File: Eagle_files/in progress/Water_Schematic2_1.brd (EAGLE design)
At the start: 26.4 x 45.5 mm, 10 parts

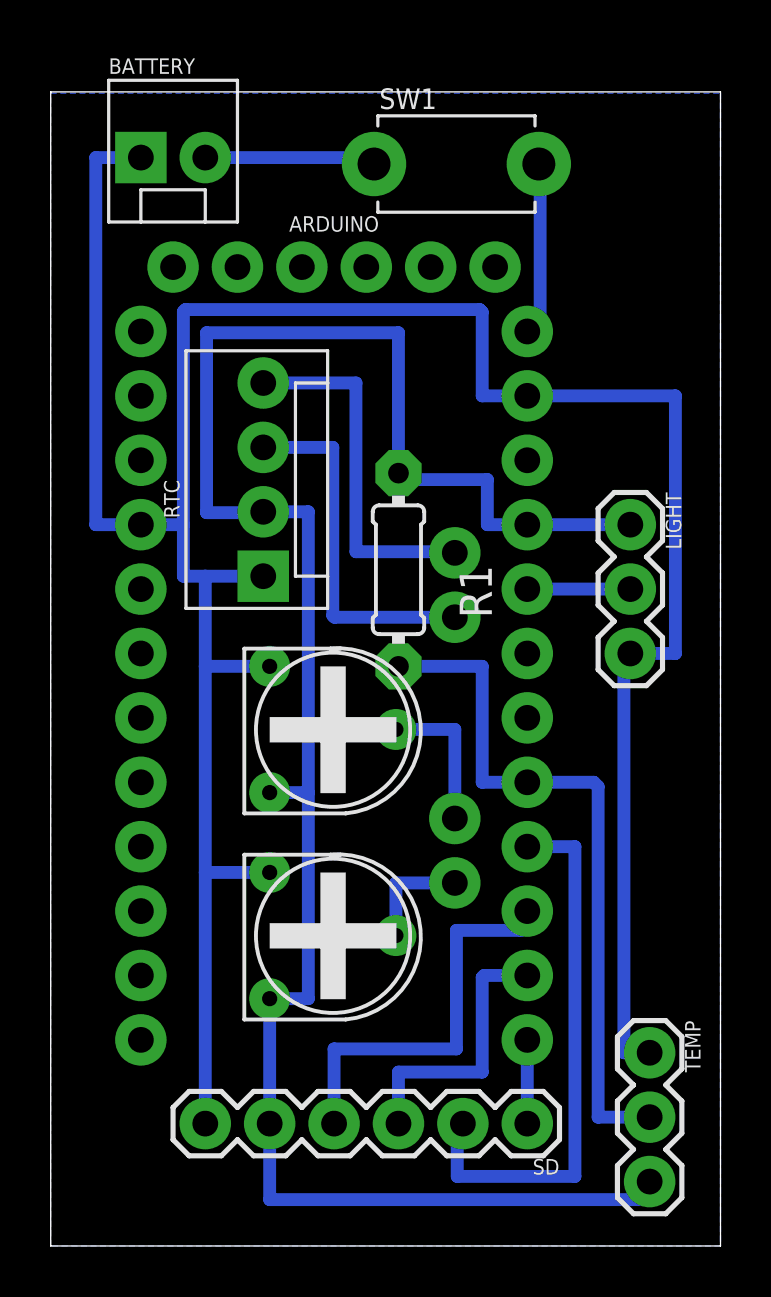
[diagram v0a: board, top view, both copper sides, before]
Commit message: updating readme
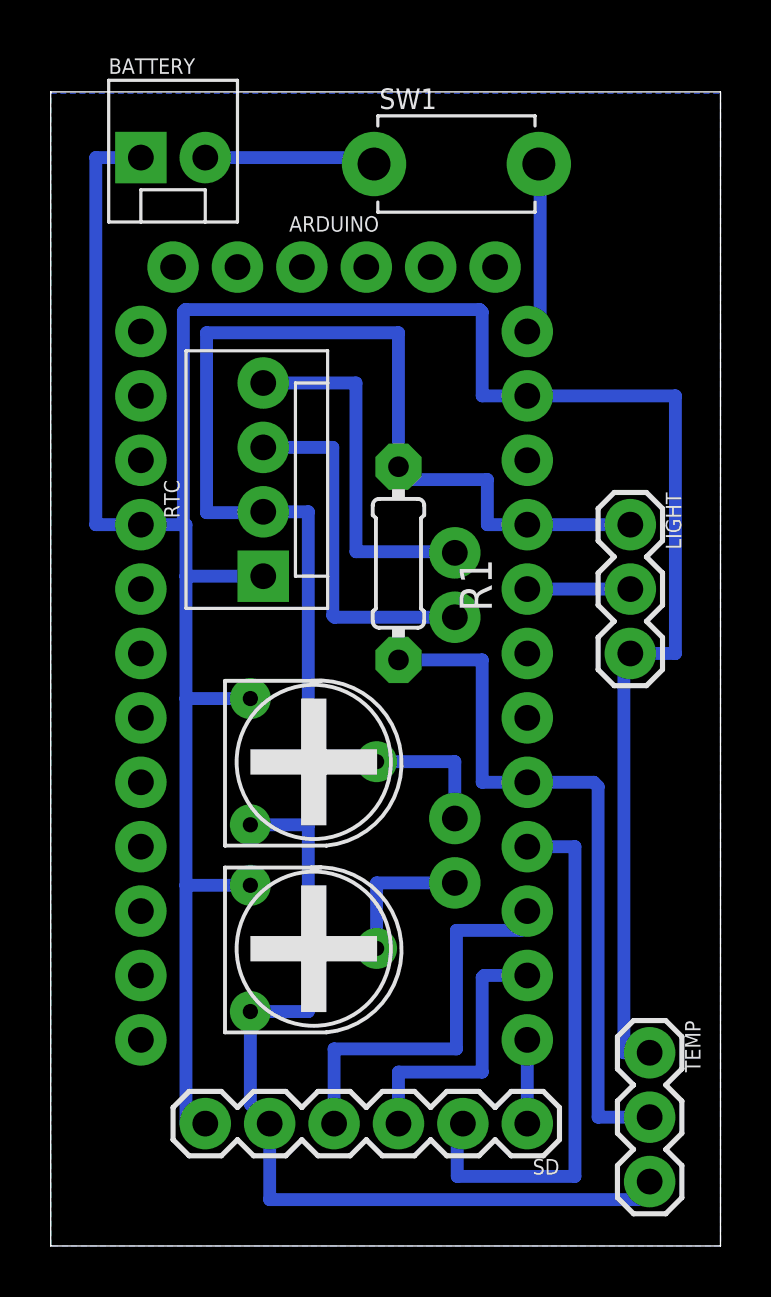
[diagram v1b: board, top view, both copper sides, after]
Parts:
- moved POT2 1.48 mm to (7.87, 21.6)
- moved POT1 0.92 mm to (7.87, 14.2)
- moved R1 0.25 mm to (13.7, 26.9)
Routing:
- net VCC: track 81.0 -> 82.7 mm
- net A6: track 4.40 -> 5.67 mm
- net GND: track 111.0 -> 111.8 mm
- net A7: track 5.84 -> 5.33 mm
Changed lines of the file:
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@@
 </autorouter>
 <elements>
-<element name="R1" library="rcl" library_urn="urn:adsk.eagle:library:334" package="0204/7" package3d_urn="urn:adsk.eagle:package:23498/2" value="4.7K" x="13.716" y="26.67" smashed="yes" rot="R90">
-<attribute name="NAME" x="17.399" y="24.765" size="1.27" layer="25" ratio="10" rot="R90"/>
-<attribute name="POPULARITY" value="48" x="63.246" y="67.31" size="1.778" layer="27" rot="R90" display="off"/>
-<attribute name="SPICEPREFIX" value="R" x="63.246" y="67.31" size="1.778" layer="27" rot="R90" display="off"/>
-<attribute name="VALUE" x="14.4018" y="24.384" size="1.27" layer="27" ratio="10" rot="R90"/>
+<element name="R1" library="rcl" library_urn="urn:adsk.eagle:library:334" package="0204/7" package3d_urn="urn:adsk.eagle:package:23498/2" value="4.7K" x="13.716" y="26.924" smashed="yes" rot="R90">
+<attribute name="NAME" x="17.399" y="25.019" size="1.27" layer="25" ratio="10" rot="R90"/>
+<attribute name="POPULARITY" value="48" x="63.246" y="67.564" size="1.778" layer="27" rot="R90" display="off"/>
+<attribute name="SPICEPREFIX" value="R" x="63.246" y="67.564" size="1.778" layer="27" rot="R90" display="off"/>
+<attribute name="VALUE" x="14.4018" y="24.638" size="1.27" layer="27" ratio="10" rot="R90"/>
 </element>
 <element name="ARDUINO" library="SparkFun-Boards" library_urn="urn:adsk.eagle:library:509" package="ARDUINO_PRO_MINI" package3d_urn="urn:adsk.eagle:package:37322/1" value="ARDUINO_PRO_MINI" x="11.176" y="23.368" smashed="yes">
@@
 <attribute name="VALUE" x="2.286" y="40.132" size="0.6096" layer="27" font="vector" ratio="20" align="top-left"/>
 </element>
-<element name="POT1" library="RM_065" package="RM_065" value="RM_065" x="8.636" y="14.732" smashed="yes" rot="R270"/>
-<element name="POT2" library="RM_065" package="RM_065" value="RM_065" x="8.636" y="22.86" smashed="yes" rot="R270"/>
+<element name="POT1" library="RM_065" package="RM_065" value="RM_065" x="7.874" y="14.224" smashed="yes" rot="R270"/>
+<element name="POT2" library="RM_065" package="RM_065" value="RM_065" x="7.874" y="21.59" smashed="yes" rot="R270"/>
 </elements>
 <signals>
@@
 <wire x1="23.622" y1="5.08" x2="21.59" y2="5.08" width="0.508" layer="16"/>
 <wire x1="21.59" y1="5.08" x2="21.59" y2="18.11879375" width="0.508" layer="16"/>
-<wire x1="13.716" y1="22.86" x2="17.018" y2="22.86" width="0.508" layer="16"/>
-<wire x1="17.018" y1="22.86" x2="17.018" y2="18.288" width="0.508" layer="16"/>
+<wire x1="13.716" y1="23.114" x2="17.018" y2="23.114" width="0.508" layer="16"/>
+<wire x1="17.018" y1="23.114" x2="17.018" y2="18.288" width="0.508" layer="16"/>
 <wire x1="17.018" y1="18.288" x2="18.796" y2="18.288" width="0.508" layer="16"/>
 </signal>
@@
 <wire x1="3.556" y1="28.448" x2="1.778" y2="28.448" width="0.508" layer="16"/>
 <wire x1="5.31719375" y1="36.9316" x2="5.2324" y2="36.84680625" width="0.508" layer="16"/>
-<wire x1="5.2324" y1="26.416" x2="6.096" y2="26.416" width="0.508" layer="16"/>
-<wire x1="6.096" y1="26.416" x2="8.382" y2="26.416" width="0.508" layer="16"/>
+<wire x1="5.334" y1="26.416" x2="8.382" y2="26.416" width="0.508" layer="16"/>
 <wire x1="5.2324" y1="36.84680625" x2="5.2324" y2="28.448" width="0.508" layer="16"/>
-<wire x1="5.2324" y1="28.448" x2="5.2324" y2="26.416" width="0.508" layer="16"/>
+<wire x1="5.334" y1="28.448" x2="5.334" y2="26.416" width="0.508" layer="16"/>
 <wire x1="3.556" y1="28.448" x2="5.2324" y2="28.448" width="0.508" layer="16"/>
-<wire x1="6.096" y1="4.826" x2="6.096" y2="14.732" width="0.508" layer="16"/>
-<wire x1="6.096" y1="14.732" x2="6.096" y2="22.86" width="0.508" layer="16"/>
-<wire x1="6.096" y1="22.86" x2="6.096" y2="26.416" width="0.508" layer="16"/>
-<wire x1="8.636" y1="22.86" x2="6.096" y2="22.86" width="0.508" layer="16"/>
-<wire x1="8.636" y1="14.732" x2="6.096" y2="14.732" width="0.508" layer="16"/>
+<wire x1="5.2324" y1="28.448" x2="5.334" y2="28.448" width="0.508" layer="16"/>
+<wire x1="5.334" y1="14.224" x2="5.334" y2="4.826" width="0.508" layer="16"/>
+<wire x1="6.096" y1="4.826" x2="5.334" y2="4.826" width="0.508" layer="16"/>
+<wire x1="5.334" y1="14.224" x2="5.334" y2="21.59" width="0.508" layer="16"/>
+<wire x1="5.334" y1="21.59" x2="5.334" y2="26.416" width="0.508" layer="16"/>
+<wire x1="7.874" y1="21.59" x2="5.334" y2="21.59" width="0.508" layer="16"/>
+<wire x1="7.874" y1="14.224" x2="5.334" y2="14.224" width="0.508" layer="16"/>
 <wire x1="18.796" y1="33.528" x2="19.304" y2="33.528" width="0" layer="19" extent="16-16"/>
 </signal>
@@
 <contactref element="TEMP" pad="3"/>
 <contactref element="RTC" pad="2"/>
-<wire x1="17.2212" y1="30.226" x2="13.97" y2="30.226" width="0.508" layer="16"/>
-<wire x1="13.716" y1="30.48" x2="13.97" y2="30.226" width="0.508" layer="16"/>
+<wire x1="17.2212" y1="30.226" x2="14.224" y2="30.226" width="0.508" layer="16"/>
+<wire x1="13.716" y1="30.734" x2="14.224" y2="30.226" width="0.508" layer="16"/>
 <wire x1="8.636" y1="1.8288" x2="8.636" y2="4.826" width="0.508" layer="16"/>
 <contactref element="POT2" pad="VCC"/>
 <contactref element="POT1" pad="VCC"/>
-<wire x1="13.716" y1="30.48" x2="13.716" y2="36.0172" width="0.508" layer="16"/>
+<wire x1="13.716" y1="30.734" x2="13.716" y2="36.0172" width="0.508" layer="16"/>
 <wire x1="13.716" y1="36.0172" x2="6.1468" y2="36.0172" width="0.508" layer="16"/>
 <wire x1="6.1468" y1="28.92200625" x2="6.1468" y2="36.0172" width="0.508" layer="16"/>
@@
 <wire x1="17.2212" y1="28.448" x2="18.796" y2="28.448" width="0.508" layer="16"/>
 <wire x1="22.86" y1="28.448" x2="18.796" y2="28.448" width="0.508" layer="16"/>
-<wire x1="8.636" y1="9.7536" x2="10.16" y2="9.7536" width="0.508" layer="16"/>
-<wire x1="10.16" y1="9.7536" x2="10.16" y2="17.8816" width="0.508" layer="16"/>
-<wire x1="8.636" y1="4.826" x2="8.636" y2="9.7536" width="0.508" layer="16"/>
-<wire x1="10.16" y1="17.8816" x2="8.636" y2="17.8816" width="0.508" layer="16"/>
-<wire x1="10.16" y1="28.956" x2="10.16" y2="17.8816" width="0.508" layer="16"/>
+<wire x1="7.874" y1="9.2456" x2="10.16" y2="9.2456" width="0.508" layer="16"/>
+<wire x1="10.16" y1="9.2456" x2="10.16" y2="16.6116" width="0.508" layer="16"/>
+<wire x1="7.874" y1="9.2456" x2="7.874" y2="5.588" width="0.508" layer="16"/>
+<wire x1="8.636" y1="4.826" x2="7.874" y2="5.588" width="0.508" layer="16"/>
+<wire x1="10.16" y1="16.6116" x2="7.874" y2="16.6116" width="0.508" layer="16"/>
+<wire x1="10.16" y1="28.956" x2="10.16" y2="16.6116" width="0.508" layer="16"/>
 </signal>
 <signal name="SDA">
@@
 <contactref element="ARDUINO" pad="A6"/>
 <contactref element="POT1" pad="OUT"/>
-<wire x1="15.9385" y1="14.31925" x2="13.6144" y2="14.31925" width="0.508" layer="16"/>
-<wire x1="13.6144" y1="14.31925" x2="13.6144" y2="12.2428" width="0.508" layer="16"/>
+<wire x1="15.9385" y1="14.31925" x2="12.8524" y2="14.31925" width="0.508" layer="16"/>
+<wire x1="12.8524" y1="14.31925" x2="12.8524" y2="11.7348" width="0.508" layer="16"/>
 </signal>
 <signal name="A7">
 <contactref element="ARDUINO" pad="A7"/>
 <contactref element="POT2" pad="OUT"/>
-<wire x1="15.9385" y1="16.85925" x2="15.9385" y2="20.3708" width="0.508" layer="16"/>
-<wire x1="15.9385" y1="20.3708" x2="13.6144" y2="20.3708" width="0.508" layer="16"/>
+<wire x1="15.9385" y1="16.85925" x2="15.9385" y2="19.1008" width="0.508" layer="16"/>
+<wire x1="15.9385" y1="19.1008" x2="12.8524" y2="19.1008" width="0.508" layer="16"/>
 </signal>
 </signals>
